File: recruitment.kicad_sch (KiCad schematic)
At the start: 26 parts, among them K1 Panasonic_ALFG2PF091, Q1 IRF9540N, Q2 BC337, Q3 BC327, U1 LM7805_TO220, U2 OP275, U3 OP275, U4 74LVC1G373

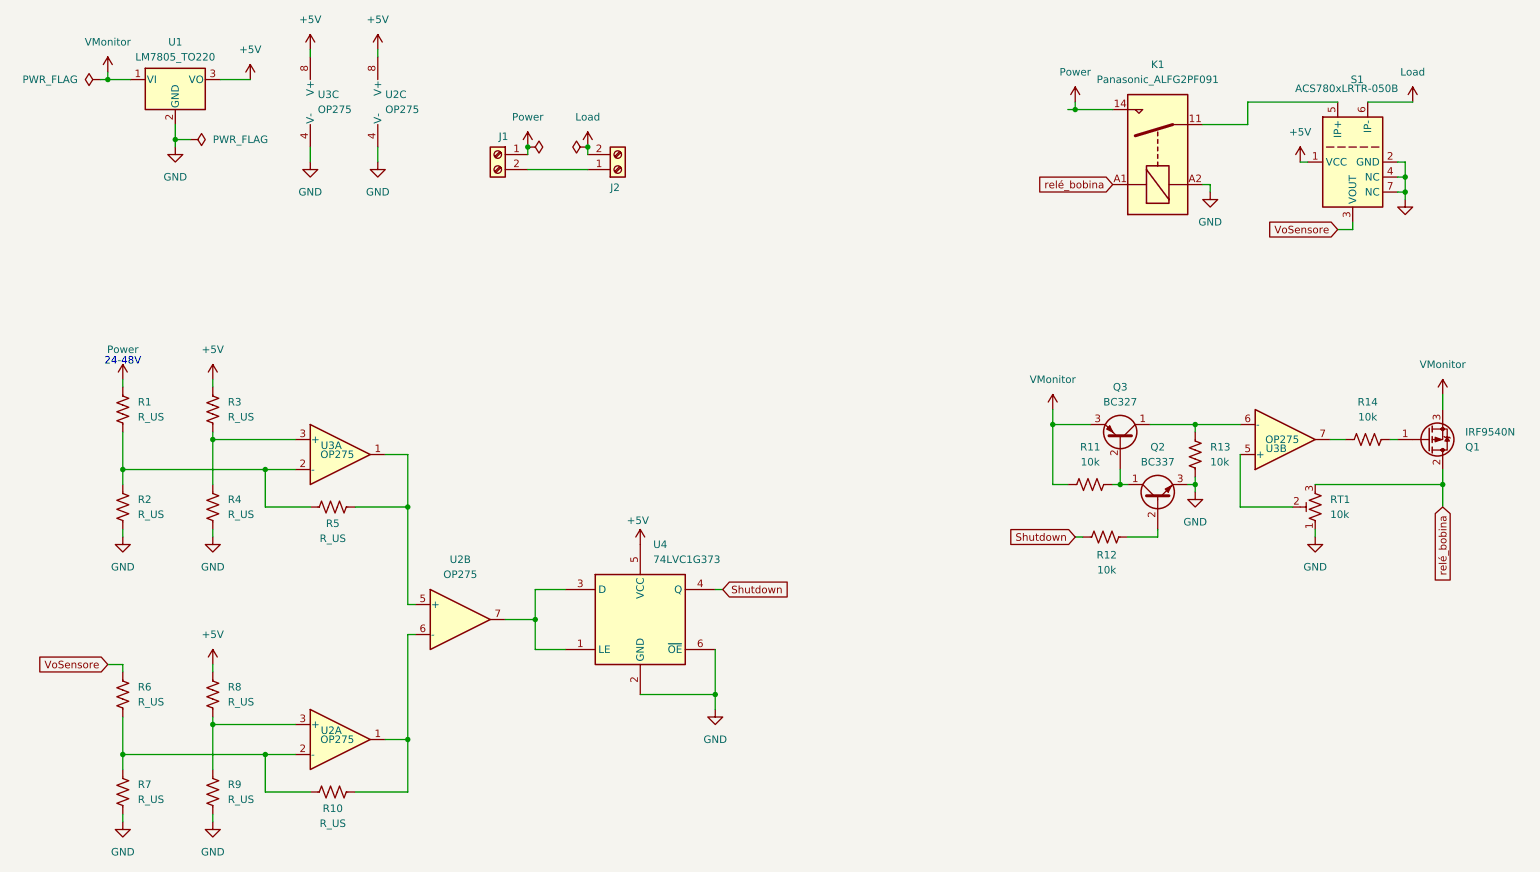
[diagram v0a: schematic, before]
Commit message: V1.0.0 : prima versione (si spera) funzionante
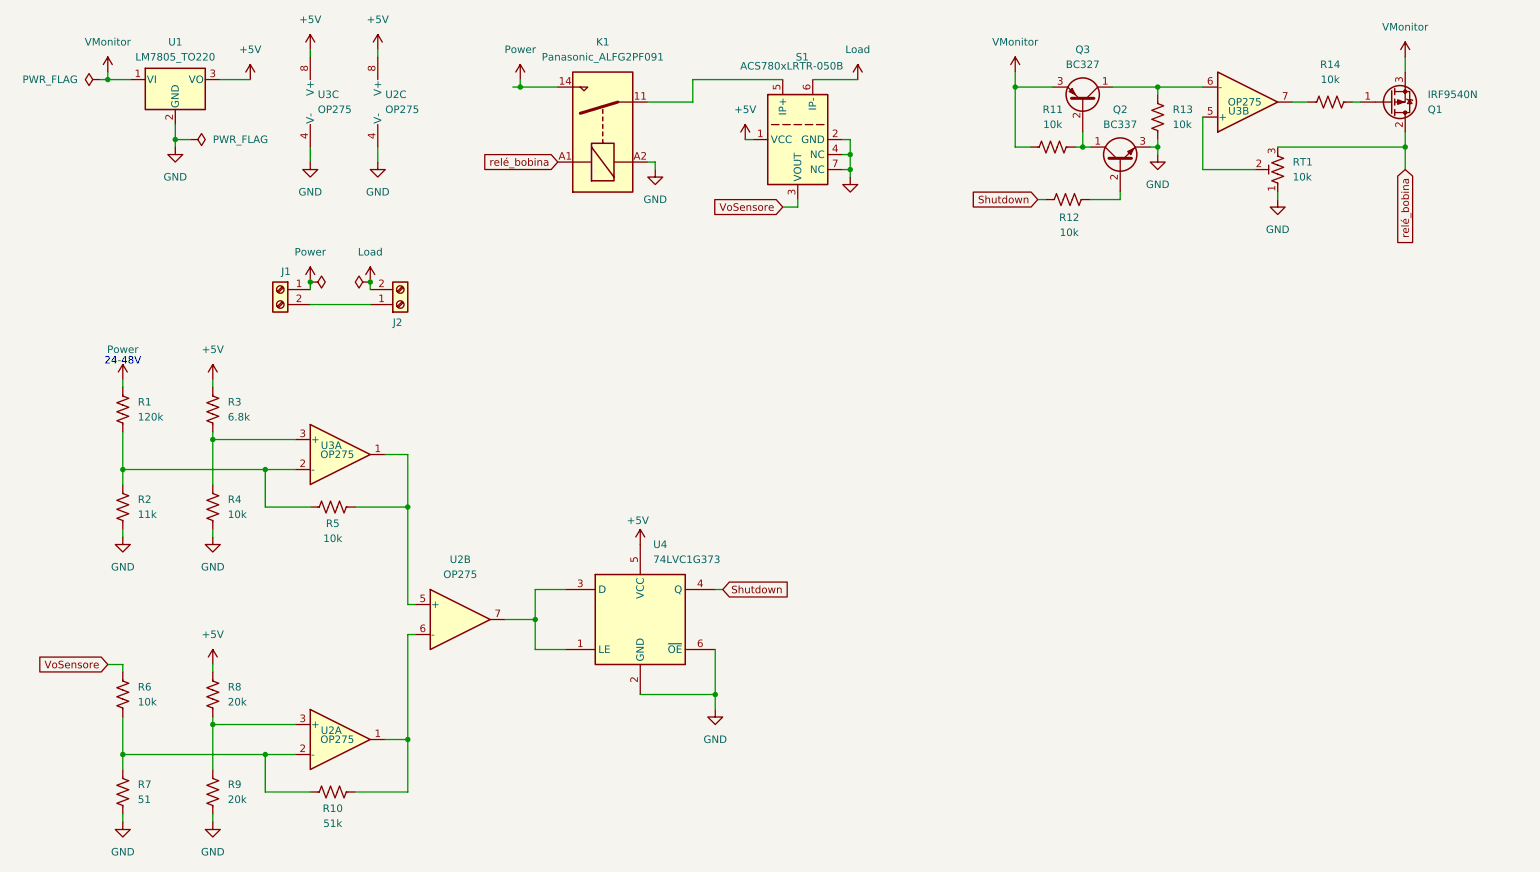
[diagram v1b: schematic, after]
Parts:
- R1: value R_US -> 120k
- R10: value R_US -> 51k
- R2: value R_US -> 11k
- R3: value R_US -> 6.8k
- R4, R5, R6: value R_US -> 10k
- R7: value R_US -> 51
- R8, R9: value R_US -> 20k
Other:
- title: Template -> Test d'ingresso
- moved on the sheet: J1, J2, K1, Q1, Q2, Q3, R11, R12, R13, R14, RT1, S1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
